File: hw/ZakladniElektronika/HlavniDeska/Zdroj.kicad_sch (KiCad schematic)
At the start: 28 parts, among them Q10 Q_PMOS_DGS-L, SW1 ON, U17 BateriCell_2x, U7 SL8261D-G3JE

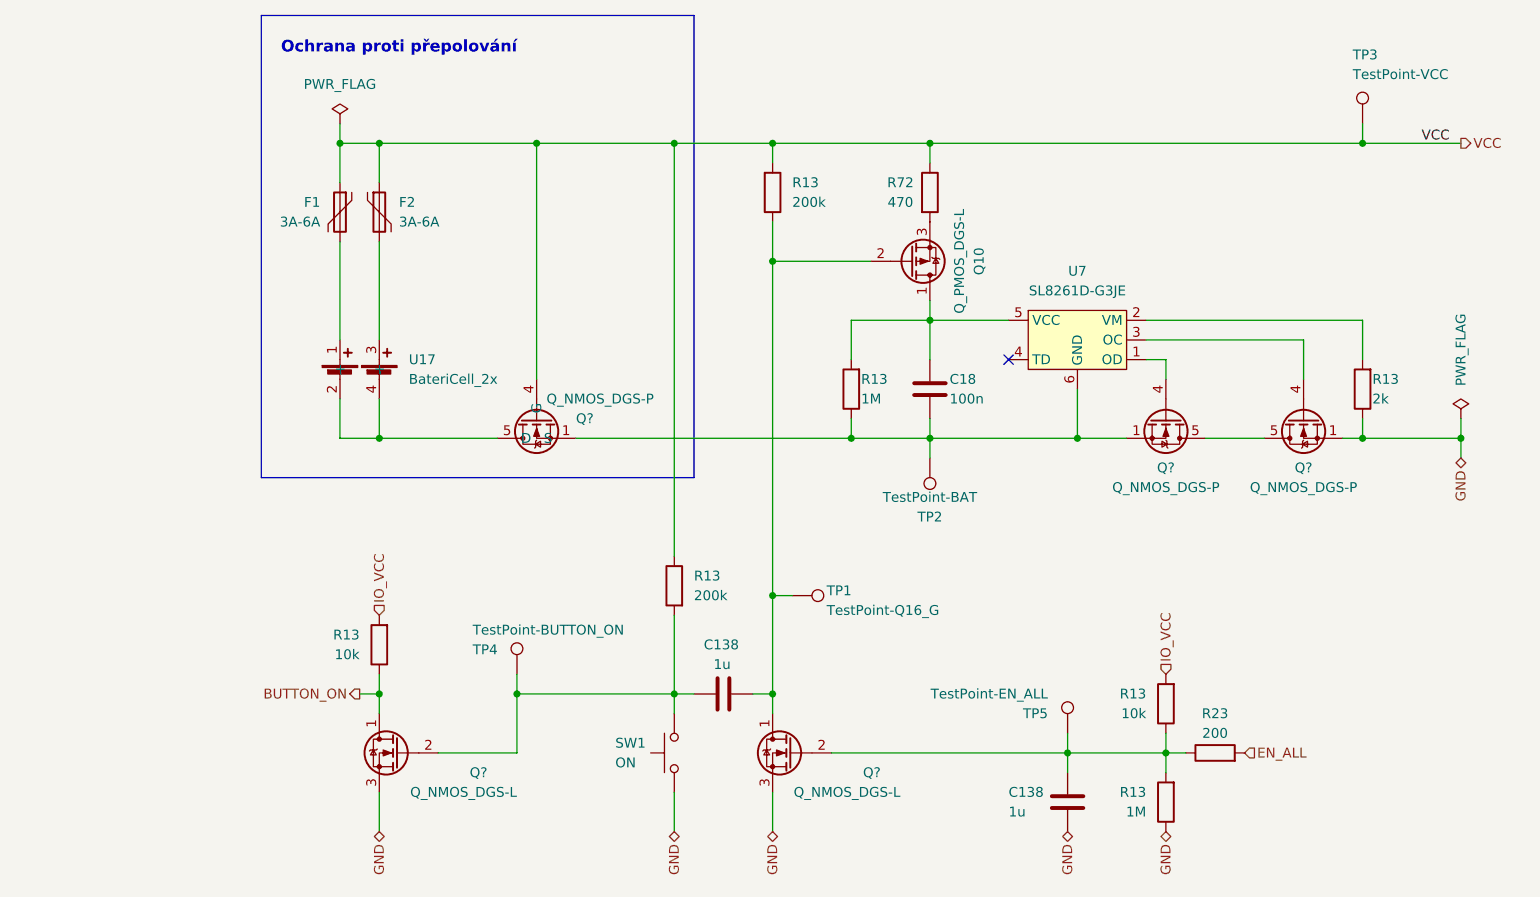
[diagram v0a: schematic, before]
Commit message: WPI (zápínací logika)
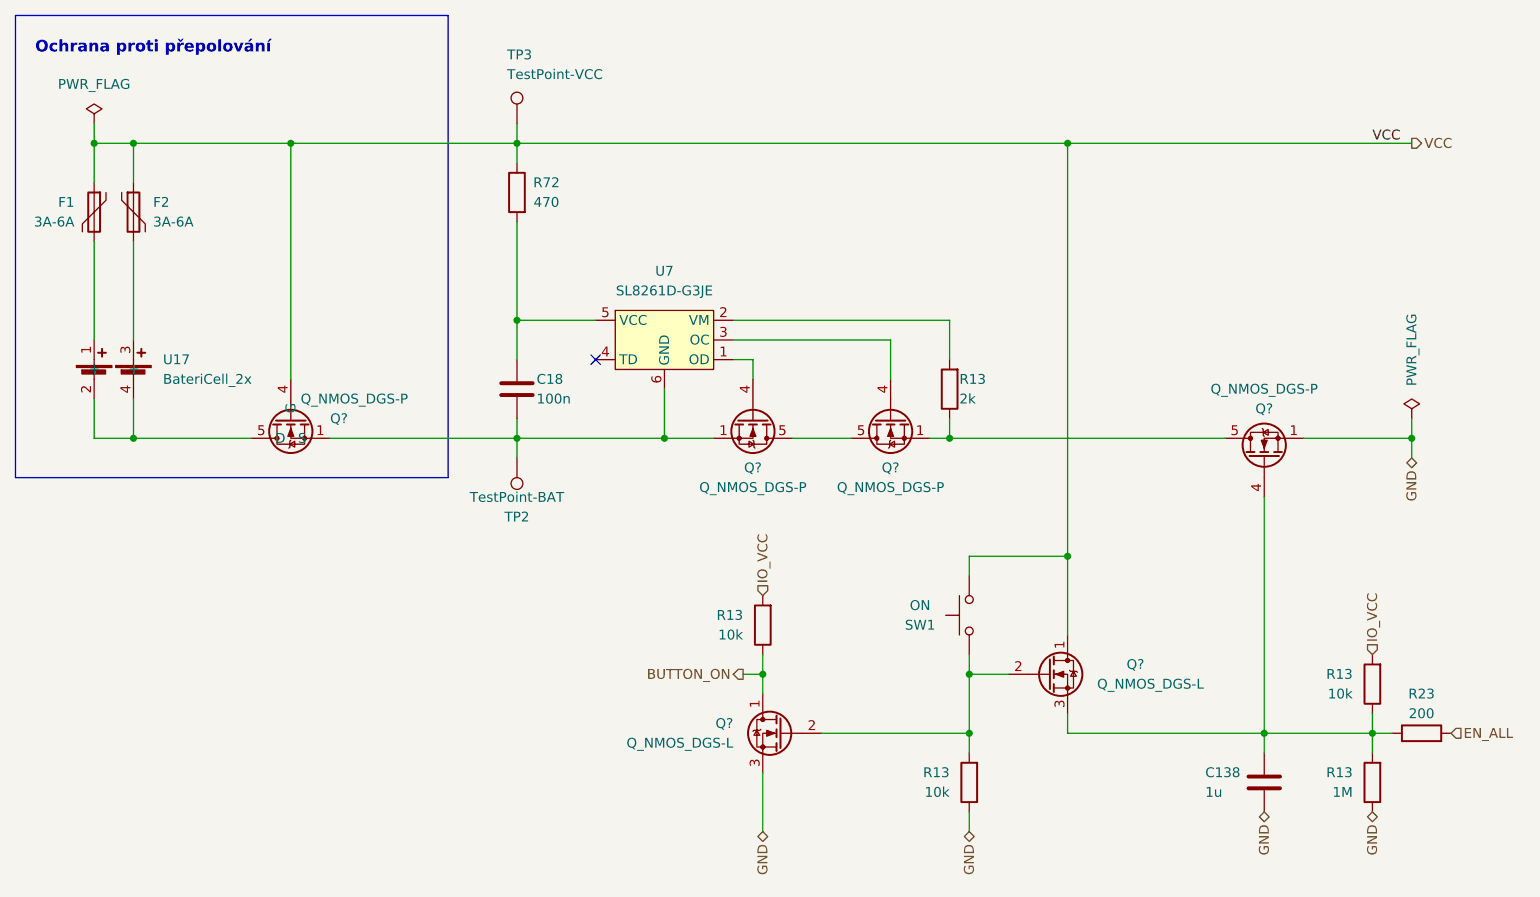
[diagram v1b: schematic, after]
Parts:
- removed C138: 1u, Capacitor_SMD:C_0402_1005Metric, symbol Device:C
- removed Q10: Q_PMOS_DGS-L, Package_TO_SOT_SMD:SOT-23, symbol Device:Q_PMOS_DGS
- removed Q?: Q_NMOS_DGS-L, Package_TO_SOT_SMD:SOT-23, symbol Device:Q_NMOS_DGS
- removed R13: 1M, Resistor_SMD:R_0402_1005Metric, symbol Device:R
- removed R13 (x2): 200k, Resistor_SMD:R_0402_1005Metric, symbol Device:R
- removed TP1: TestPoint-Q16_G, Connector_Pin:Pin_D0.9mm_L10.0mm_W2.4mm_FlatFork, symbol Connector:TestPoint
- removed TP4: TestPoint-BUTTON_ON, Connector_Pin:Pin_D0.9mm_L10.0mm_W2.4mm_FlatFork, symbol Connector:TestPoint
- removed TP5: TestPoint-EN_ALL, Connector_Pin:Pin_D0.9mm_L10.0mm_W2.4mm_FlatFork, symbol Connector:TestPoint
- added Q?: Q_NMOS_DGS-P, Package_SON:Diodes_PowerDI3333-8, symbol RKL-Uncategorized:Si7112DN
- added Q?: Q_NMOS_DGS-L, Package_TO_SOT_SMD:SOT-23, symbol Device:Q_NMOS_DGS
- added R13: 10k, Resistor_SMD:R_0402_1005Metric, symbol Device:R
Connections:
- net GND: now also Q?.1 (S), Q?.2 (S), Q?.3 (S), R13.1; no longer Q?.1 (S), Q?.2 (S), Q?.3 (S), R13.1, SW1.1
- net VCC: now also SW1.1, Q?.1 (D)
- net at Q?.2 (G), SW1.2: now also Q?.2 (G), R13.2
- net at C138.1, R13.1, R13.2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: now also Q?.3 (S), Q?.4 (G)
- net at C18.1, U7.5 (VCC): now also R72.2
- new net: Q?.1 (S), Q?.2 (S), Q?.3 (S), Q?.5 (D), R13.1
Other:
- moved on the sheet: C138, C18, F1, F2, Q?, R13, R23, R72, SW1, TP2, TP3, U17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
